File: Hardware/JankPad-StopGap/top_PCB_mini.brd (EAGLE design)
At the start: 110.5 x 67.5 mm, 7 parts

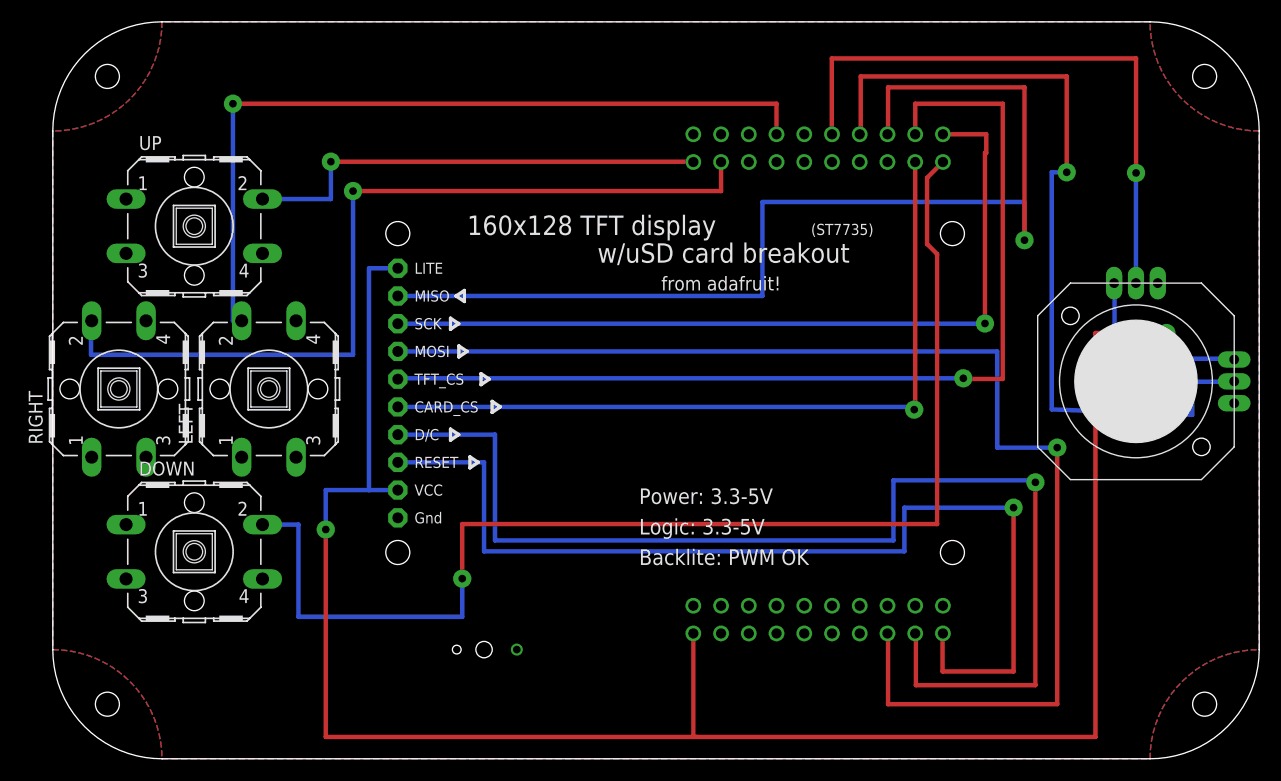
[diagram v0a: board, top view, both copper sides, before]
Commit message: Snapshot!!
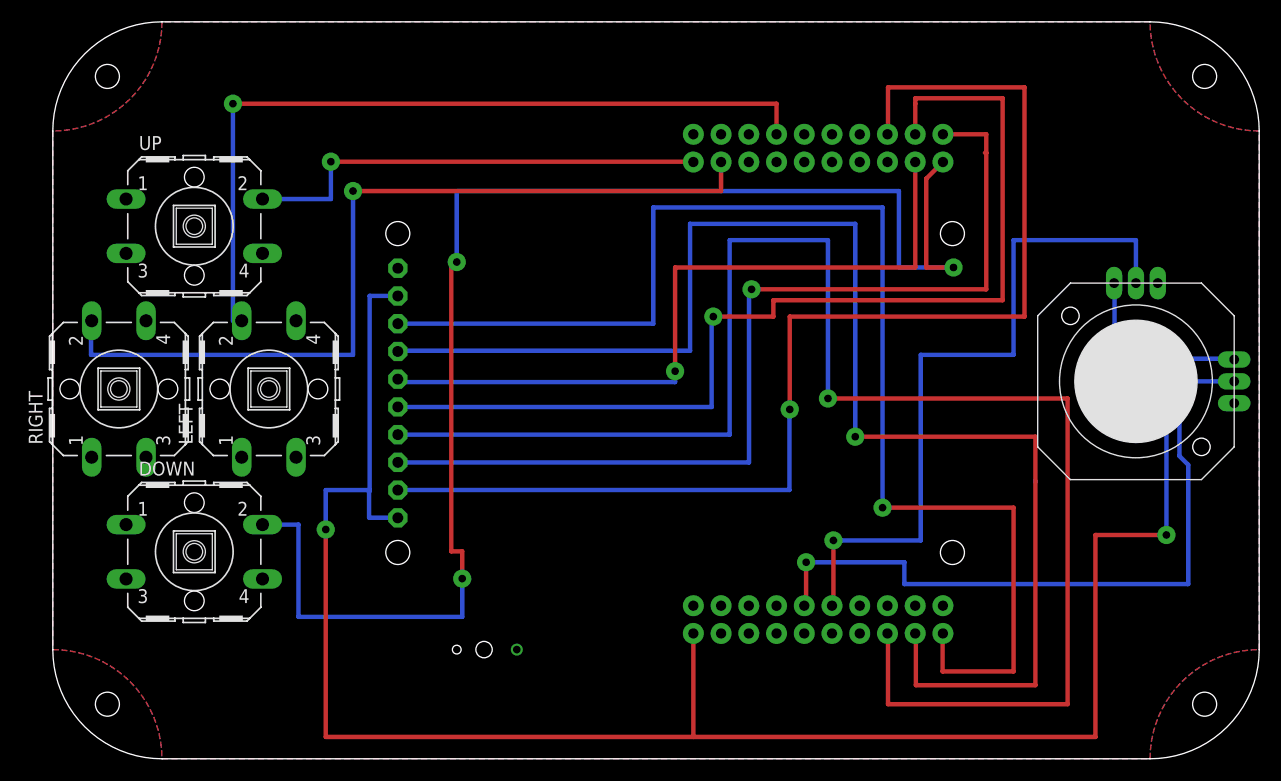
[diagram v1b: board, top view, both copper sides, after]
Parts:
- flipped DISPLAY to the bottom, turned to 180 degrees
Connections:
- removed net N$28: LAUNCHPAD.PB6, LEFTJOYSTICK.X
- removed net N$34: LAUNCHPAD.PB7, LEFTJOYSTICK.Y
- new net N$10: LAUNCHPAD.PB6
- new net N$11: LAUNCHPAD.PD2, LEFTJOYSTICK.X
- new net N$12: LAUNCHPAD.PD3, LEFTJOYSTICK.Y
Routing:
- net N$28: track 75.9 -> 0.00 mm, vias 1 -> 0
- net N$12: track 0.00 -> 65.2 mm, vias 0 -> 1
- net N$11: track 0.00 -> 64.6 mm, vias 0 -> 1
- net N$34: track 55.4 -> 0.00 mm, vias 1 -> 0
- net N$6: track 114.7 -> 144.6 mm
- net N$1: track 93.6 -> 119.6 mm
- net N$2: track 108.3 -> 128.3 mm
- net N$32: track 112.9 -> 132.5 mm, vias 1 -> 3
- net N$7: track 75.2 -> 88.1 mm
- net N$8: track 100.4 -> 111.1 mm
- net N$31: track 196.0 -> 191.3 mm
- net N$5: track 91.6 -> 95.0 mm
- net N$3: track 70.3 -> 67.8 mm
